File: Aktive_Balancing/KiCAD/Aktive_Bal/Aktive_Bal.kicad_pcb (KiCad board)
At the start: 4 copper layers, 108.8 x 101.3 mm, 219 parts, among them J1 Screw_Terminal_01x02, J10 Conn_01x02_Pin, J11 Conn_01x02_Pin, J12 Conn_01x02_Pin, J13 Conn_01x02_Pin, J14 Conn_01x02_Pin, J15 Screw_Terminal_01x03, J16 Screw_Terminal_01x03, J17 Screw_Terminal_01x03, J18 Screw_Terminal_01x03, J19 Screw_Terminal_01x03, J2 A-DF_09_A_KG-T4S, J20 Screw_Terminal_01x03, J21 Conn_01x02_Pin, J22 Conn_01x02_Pin, J23 Conn_01x02_Pin, J24 Conn_01x02_Pin, J3 Conn_01x02_Pin, J4 Conn_01x02_Pin, J5 Conn_01x02_Pin, J6 Conn_01x02_Pin, J7 Sockel_BluePill, J9 Conn_01x02_Pin, Q1 BSS316NH6327XTSA1, Q10_H1 NTTFS6H888NL, Q10_L1 NTTFS6H888NL, Q11_H1 NTTFS6H888NL, Q11_L1 NTTFS6H888NL, Q12_H1 NTTFS6H888NL, Q12_L1 NTTFS6H888NL, Q13_H1 NTTFS6H888NL, Q13_L1 NTTFS6H888NL, Q14_H1 NTTFS6H888NL, Q14_L1 NTTFS6H888NL, Q15_H1 NTTFS6H888NL, Q15_L1 NTTFS6H888NL, Q16_H1 NTTFS6H888NL, Q16_L1 NTTFS6H888NL, Q1_H1 NTTFS6H888NL, Q1_L1 NTTFS6H888NL, Q2_H1 NTTFS6H888NL, Q2_L1 NTTFS6H888NL, Q3_H1 NTTFS6H888NL, Q3_L1 NTTFS6H888NL, Q4_H1 NTTFS6H888NL, Q4_L1 NTTFS6H888NL, Q5_H1 NTTFS6H888NL, Q5_L1 NTTFS6H888NL, Q6_H1 NTTFS6H888NL, Q6_L1 NTTFS6H888NL, Q7_H1 NTTFS6H888NL, Q7_L1 NTTFS6H888NL, Q8_H1 NTTFS6H888NL, Q8_L1 NTTFS6H888NL, Q9_H1 NTTFS6H888NL, Q9_L1 NTTFS6H888NL, U1 RFP12N10L, U10 LTV-847S, U11 LTV-847S, U12 LTV-847S, U13 LTV-847S, U14 TL084, U15 LM2596S-ADJ, U2 ADUM1250ARZ-RL7, U3 SN65HVD233, U4 SCW20C-12, U5 EC1SA16N, U6 PCA9306DC, U7 PCF8575CDB, U8 LM1117MP-3.3, U9 MCP4725xxx-xCH

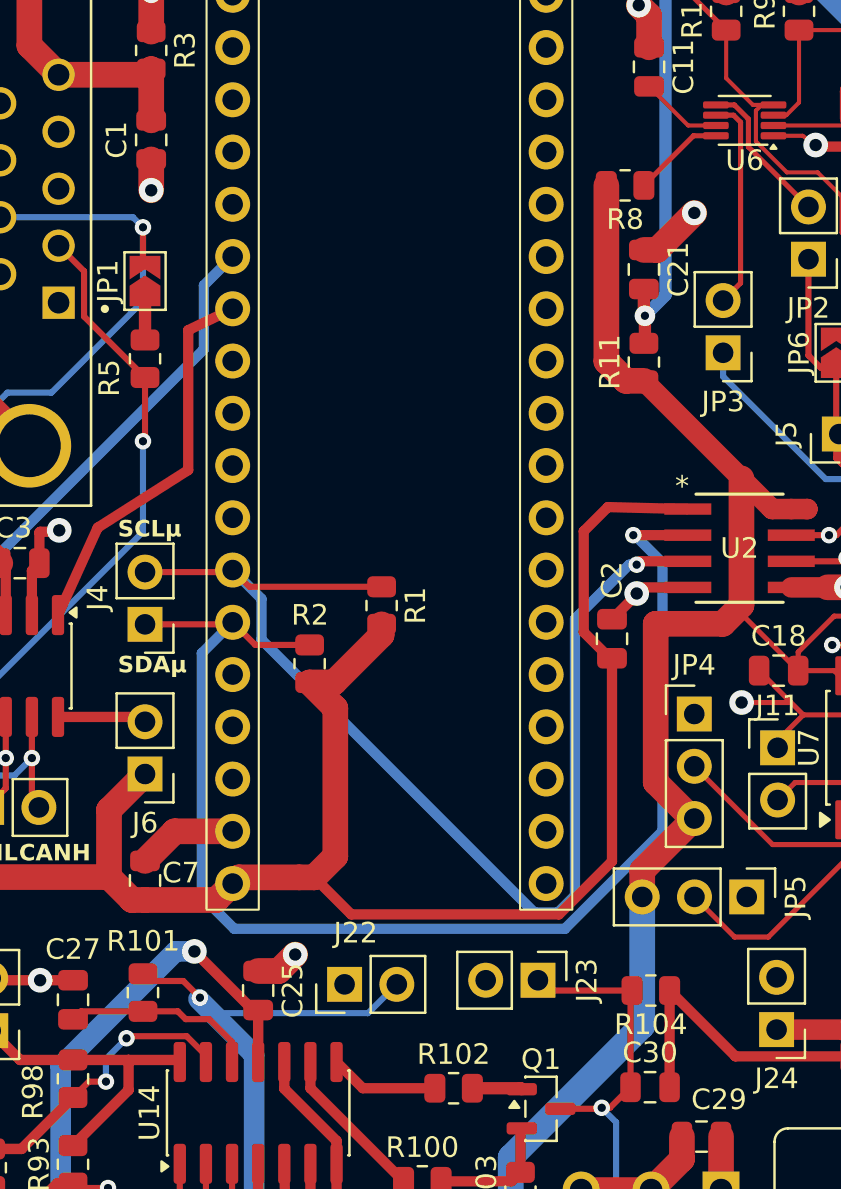
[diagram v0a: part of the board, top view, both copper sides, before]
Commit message: qwert
qer
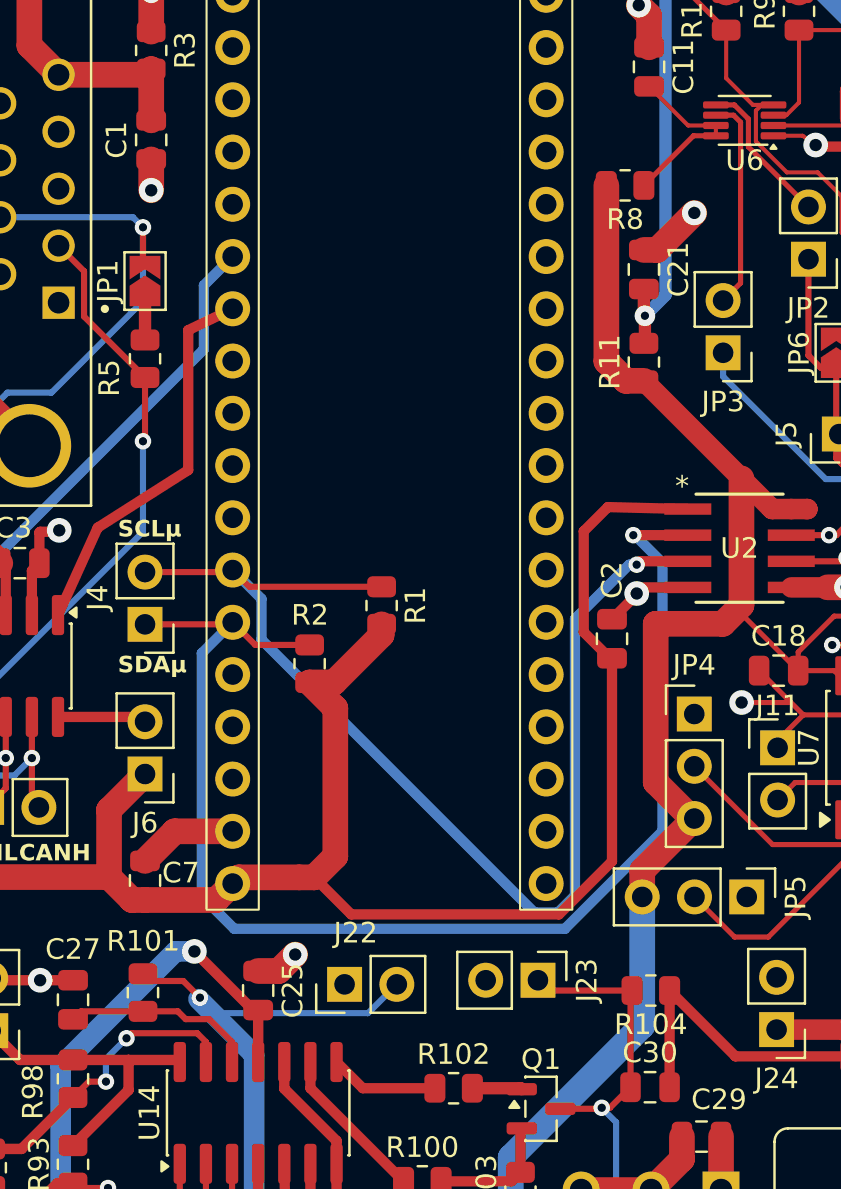
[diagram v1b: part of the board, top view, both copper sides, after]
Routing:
- net Net-(U14D--): track 14.1 -> 14.6 mm
- net Net-(U6-EN): track 8.54 -> 9.04 mm
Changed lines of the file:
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@@
 	)
 	(segment
-		(start 134.5 82)
-		(end 137 79.5)
-		(width 0.508)
+		(start 139.846 76.375)
+		(end 143.034999 76.375)
+		(width 0.3)
 		(layer "F.Cu")
 		(net "Net-(U14D--)")
 	)
 	(segment
-		(start 143.46 77.775)
-		(end 143.46 77.457732)
-		(width 0.3)
+		(start 134.5 82)
+		(end 137 79.5)
+		(width 0.508)
 		(layer "F.Cu")
 		(net "Net-(U14D--)")
@@
 	)
 	(segment
-		(start 142.522268 76.52)
-		(end 139.701 76.52)
+		(start 143.034999 76.375)
+		(end 143.46 76.800001)
 		(width 0.3)
 		(layer "F.Cu")
@@
 	)
 	(segment
-		(start 143.46 77.457732)
-		(end 142.522268 76.52)
+		(start 143.46 76.800001)
+		(end 143.46 77.775)
 		(width 0.3)
 		(layer "F.Cu")
@@
 	)
 	(segment
-		(start 139.701 76.52)
-		(end 139.6 76.621)
+		(start 139.6 76.621)
+		(end 139.846 76.375)
 		(width 0.3)
 		(layer "F.Cu")
@@
 	)
 	(segment
+		(start 168.25 32.25)
+		(end 168.25 32.75)
+		(width 0.2)
+		(layer "F.Cu")
+		(net "Net-(U6-EN)")
+	)
+	(segment
 		(start 167.1625 32.75)
 		(end 164.75 35.1625)
@@
 		(polygon
 			(pts
+				(xy 179.589851 45.304) (xy 172.289851 45.304) (xy 172.289851 41.304) (xy 179.589851 41.304)
+			)
+		)
+	)
+	(zone
+		(layer "F.Cu")
+		(name "FeinPitchZone")
+		(hatch edge 0.5)
+		(connect_pads
+			(clearance 0)
+		)
+		(min_thickness 0.25)
+		(keepout
+			(tracks allowed)
+			(vias allowed)
+			(pads allowed)
+			(copperpour allowed)
+			(footprints allowed)
+		)
+		(placement
+			(enabled no)
+			(sheetname "/")
+		)
+		(fill
+			(thermal_gap 0.5)
+			(thermal_bridge_width 0.5)
+			(island_removal_mode 0)
+		)
+		(polygon
+			(pts
 				(xy 150.734124 84.321134) (xy 141.196852 84.321134) (xy 141.196852 76.216638) (xy 150.734124 76.216638)
 			)
 		)
+	)
+	(zone
+		(layer "F.Cu")
+		(name "FeinPitchZone")
+		(hatch edge 0.5)
+		(connect_pads
+			(clearance 0)
+		)
+		(min_thickness 0.25)
+		(keepout
+			(tracks allowed)
+			(vias allowed)
+			(pads allowed)
+			(copperpour allowed)
+			(footprints allowed)
+		)
+		(placement
+			(enabled no)
+			(sheetname "/")
+		)
+		(fill
+			(thermal_gap 0.5)
+			(thermal_bridge_width 0.5)
+			(island_removal_mode 0)
+		)
+		(polygon
+			(pts
+				(xy 142 41.304) (xy 138.7 41.304) (xy 138.7 38.304) (xy 142 38.304)
+			)
+		)
